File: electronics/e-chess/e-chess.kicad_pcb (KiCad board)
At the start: 2 copper layers, 4 parts, among them J1 WS2812_LEDs, U1 MCP23017_SP, U2 ESP32-S3

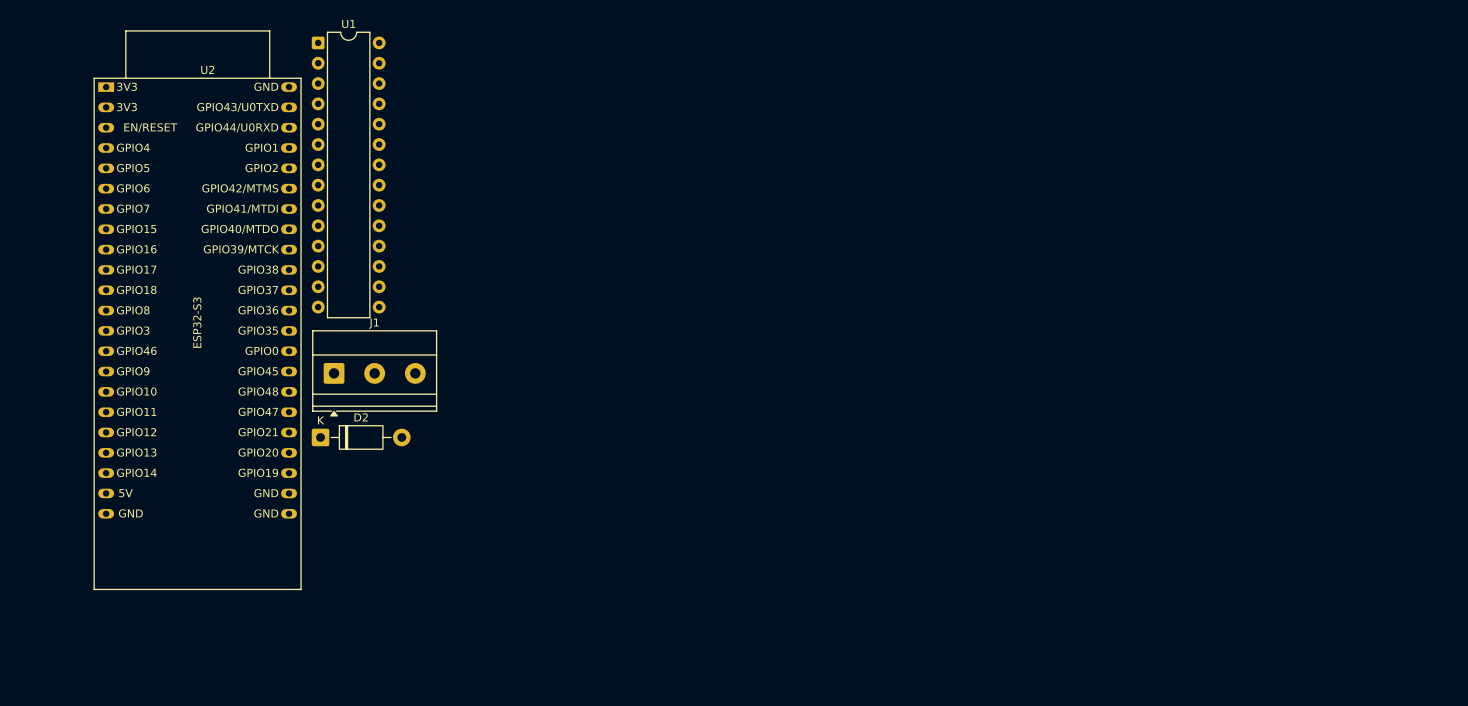
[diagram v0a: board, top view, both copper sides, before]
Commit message: Draw PCB
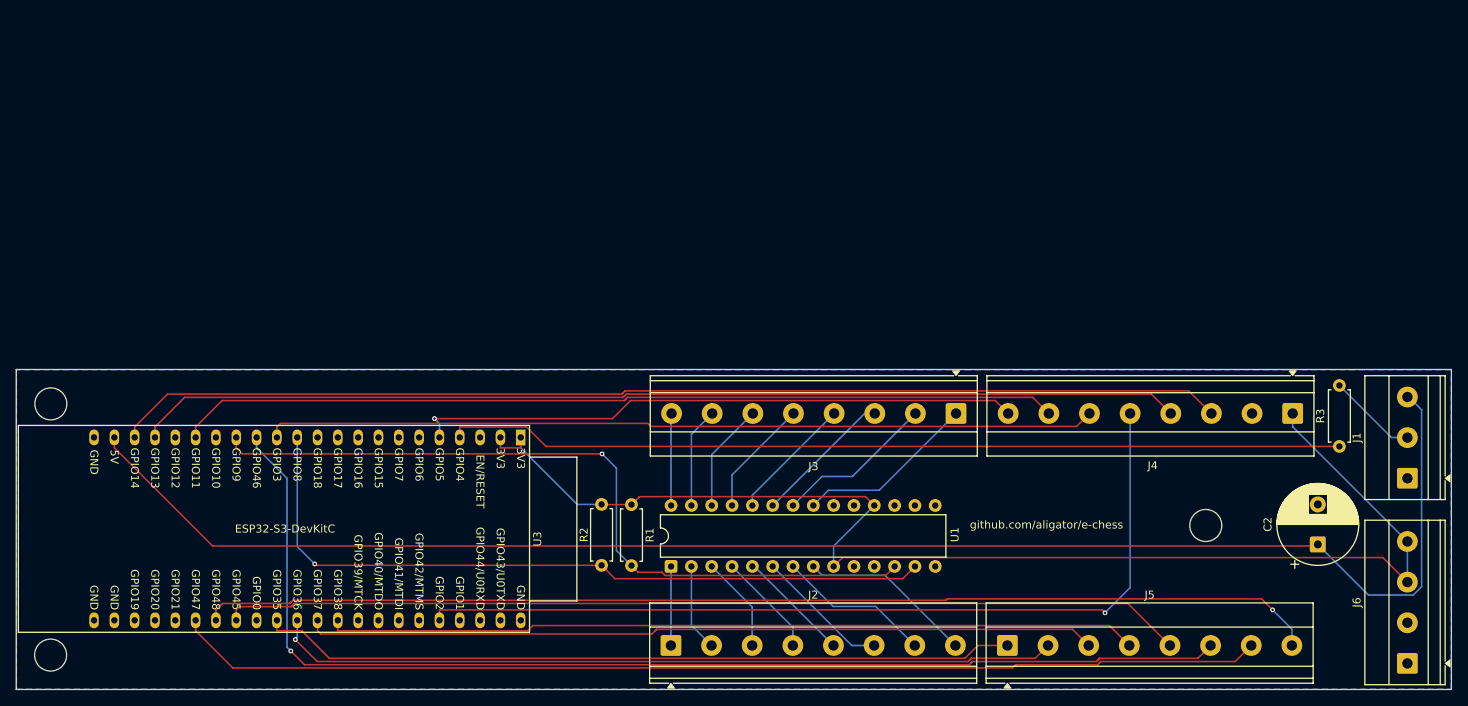
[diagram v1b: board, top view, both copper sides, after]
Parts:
- removed D2: 1N4001, Diode_THT:D_DO-41_SOD81_P10.16mm_Horizontal
- removed U2: ESP32-S3, PCM_Espressif:ESP32-S3-DevKitC
- added C2: 470 µF, Capacitor_THT:CP_Radial_D10.0mm_P5.00mm, F.Cu at (255.5, 96.4)
- added J2: Outputs, TerminalBlock_Phoenix:TerminalBlock_Phoenix_MKDS-1,5-8-5.08_1x08_P5.08mm_Horizontal, F.Cu at (174.6, 109.0)
- added J3: Inputs, TerminalBlock_Phoenix:TerminalBlock_Phoenix_MKDS-1,5-8-5.08_1x08_P5.08mm_Horizontal, F.Cu at (210.3, 80.0)
- added J4: e-Paper 1.54 inch, TerminalBlock_Phoenix:TerminalBlock_Phoenix_MKDS-1,5-8-5.08_1x08_P5.08mm_Horizontal, F.Cu at (252.4, 80.0)
- added J5: Arbitary I/O, TerminalBlock_Phoenix:TerminalBlock_Phoenix_MKDS-1,5-8-5.08_1x08_P5.08mm_Horizontal, F.Cu at (216.7, 109.0)
- added J6: Power for I/O, TerminalBlock_Phoenix:TerminalBlock_Phoenix_MKDS-1,5-4-5.08_1x04_P5.08mm_Horizontal, F.Cu at (266.7, 111.2)
- added R1: R4.7k, Resistor_THT:R_Axial_DIN0207_L6.3mm_D2.5mm_P7.62mm_Horizontal, F.Cu at (169.7, 99.0)
- added R2: R4.7k, Resistor_THT:R_Axial_DIN0207_L6.3mm_D2.5mm_P7.62mm_Horizontal, F.Cu at (166.0, 99.0)
- added R3: R470, Resistor_THT:R_Axial_DIN0207_L6.3mm_D2.5mm_P7.62mm_Horizontal, F.Cu at (258.2, 84.1)
- added REF00: MountingHole_4mm, MountingHole:MountingHole_4mm, F.Cu at (97.1, 78.8)
- added REF01: MountingHole_4mm, MountingHole:MountingHole_4mm, F.Cu at (97.1, 110.2)
- added REF02: MountingHole_4mm, MountingHole:MountingHole_4mm, F.Cu at (241.5, 94.0)
- added U3: ESP32-S3-DevKitC, PCM_Espressif:ESP32-S3-DevKitC, F.Cu at (155.9, 83.0)
- moved J1 134.8 mm to (266.7, 88.1), turned to 90 degrees
- moved U1 78.9 mm to (174.7, 99.1), turned to 90 degrees
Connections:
- J1 pad 2: unconnected-(J1-DIN-Pad2) -> Net-(J1-DIN)
- U1 pad 2: unconnected-(U1-GPB1-Pad2) -> Net-(J2-Pin_2)
- U1 pad 21: unconnected-(U1-GPA0-Pad21) -> Net-(J3-Pin_1)
- U1 pad 22: unconnected-(U1-GPA1-Pad22) -> Net-(J3-Pin_2)
- U1 pad 23: unconnected-(U1-GPA2-Pad23) -> Net-(J3-Pin_3)
- U1 pad 24: unconnected-(U1-GPA3-Pad24) -> Net-(J3-Pin_4)
- U1 pad 25: unconnected-(U1-GPA4-Pad25) -> Net-(J3-Pin_5)
- U1 pad 26: unconnected-(U1-GPA5-Pad26) -> Net-(J3-Pin_6)
- U1 pad 27: unconnected-(U1-GPA6-Pad27) -> Net-(J3-Pin_7)
- U1 pad 3: unconnected-(U1-GPB2-Pad3) -> Net-(J2-Pin_3)
- U1 pad 4: unconnected-(U1-GPB3-Pad4) -> Net-(J2-Pin_4)
- U1 pad 5: unconnected-(U1-GPB4-Pad5) -> Net-(J2-Pin_5)
- U1 pad 6: unconnected-(U1-GPB5-Pad6) -> Net-(J2-Pin_6)
- U1 pad 7: unconnected-(U1-GPB6-Pad7) -> Net-(J2-Pin_7)
- U1 pad 8: unconnected-(U1-GPB7-Pad8) -> Net-(J2-Pin_8)
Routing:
- net +5V: track 0.00 -> 197.3 mm
- net +3.3V: track 0.00 -> 164.6 mm
- net Net-(J5-GPIO46): track 0.00 -> 145.6 mm, vias 0 -> 1
- net Net-(J5-GPIO48): track 0.00 -> 140.4 mm, vias 0 -> 1
- net Net-(J4-DIN): track 0.00 -> 139.2 mm
- net Net-(J5-GPIO47): track 0.00 -> 136.8 mm
- net Net-(J4-CLK): track 0.00 -> 131.2 mm
- net Net-(J5-GPIO45): track 0.00 -> 120.8 mm
- net Net-(U3-GPIO4/ADC1_CH3): track 0.00 -> 112.3 mm
- net Net-(J4-CS): track 0.00 -> 110.9 mm, vias 0 -> 1
- net Net-(J4-RST): track 0.00 -> 110.6 mm
- net Net-(J4-DC): track 0.00 -> 103.9 mm
- net Net-(J5-GPIO38): track 0.00 -> 101.5 mm
- net Net-(J5-GPIO37): track 0.00 -> 99.2 mm
- net Net-(J5-GPIO36): track 0.00 -> 98.8 mm, vias 0 -> 1
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- added copper zone on B.Cu, net GND
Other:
- board outline added: 179.4 x 40 mm
- board text added: "github.com/aligator/e-chess"
